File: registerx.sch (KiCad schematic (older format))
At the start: 6 parts, among them U11 74LS245, U12 74LS173, U13 74LS173, U14 74LS245, U15 74LS173, U16 74LS173

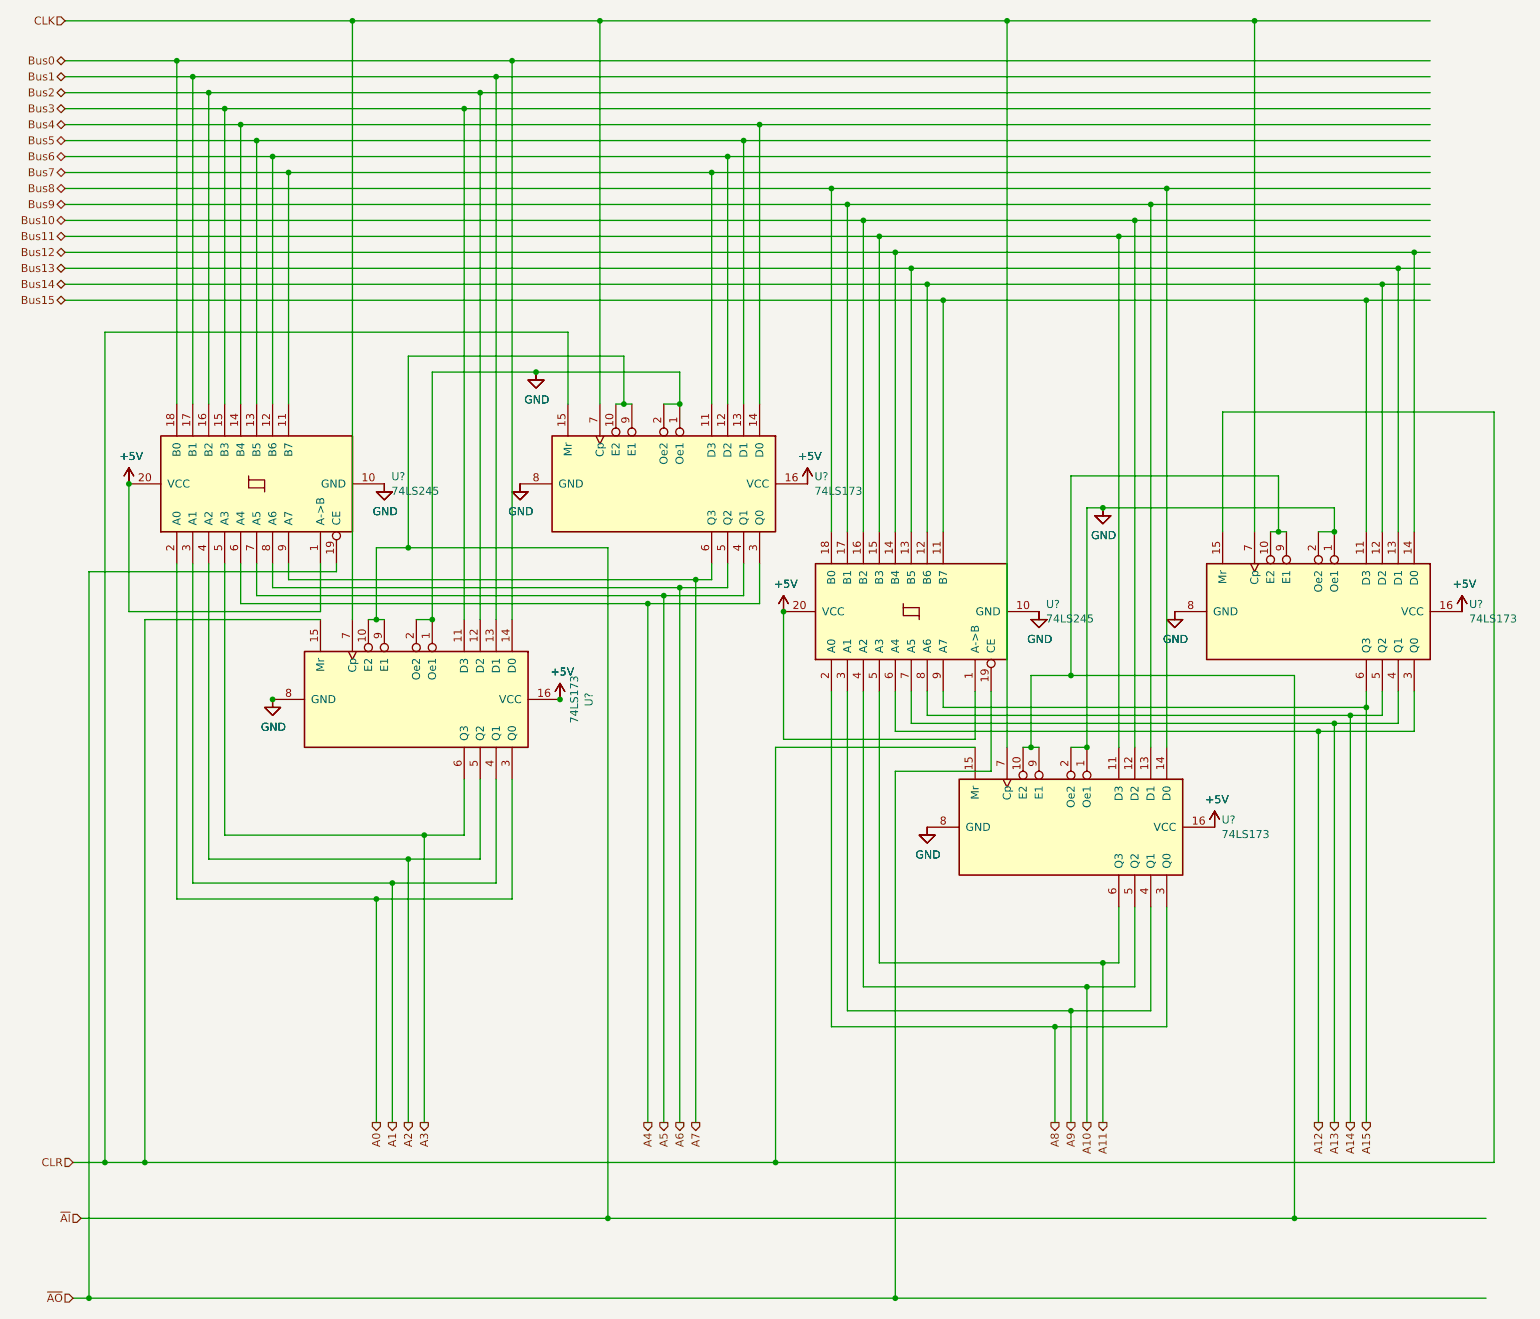
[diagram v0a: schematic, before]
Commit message: Added X register
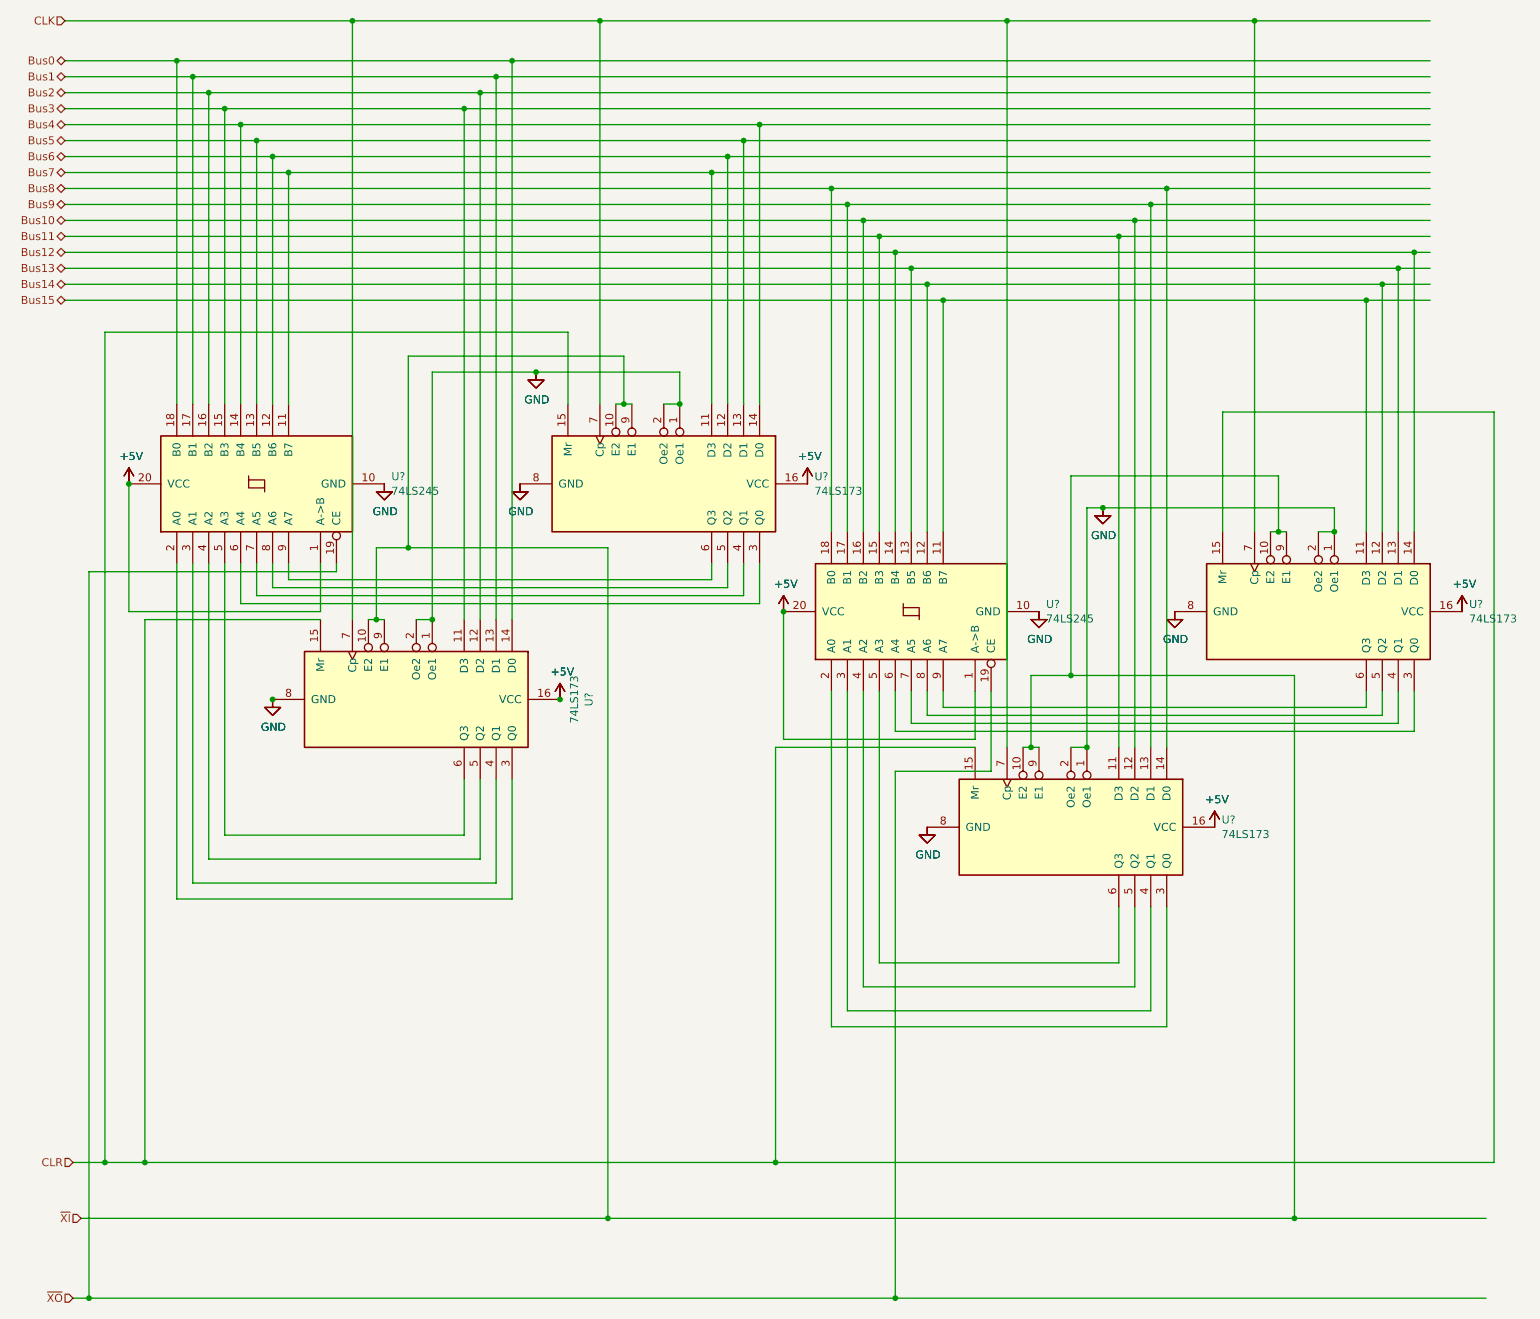
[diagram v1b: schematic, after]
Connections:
- net labels added: ~XI, ~XO
- net labels removed: A0, A1, A10, A11, A12, A13, A14, A15, A2, A3, A4, A5, A6, A7, A8, A9, ~AI, ~AO
- wire segments 234 -> 203
